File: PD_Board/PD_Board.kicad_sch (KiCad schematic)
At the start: 14 parts

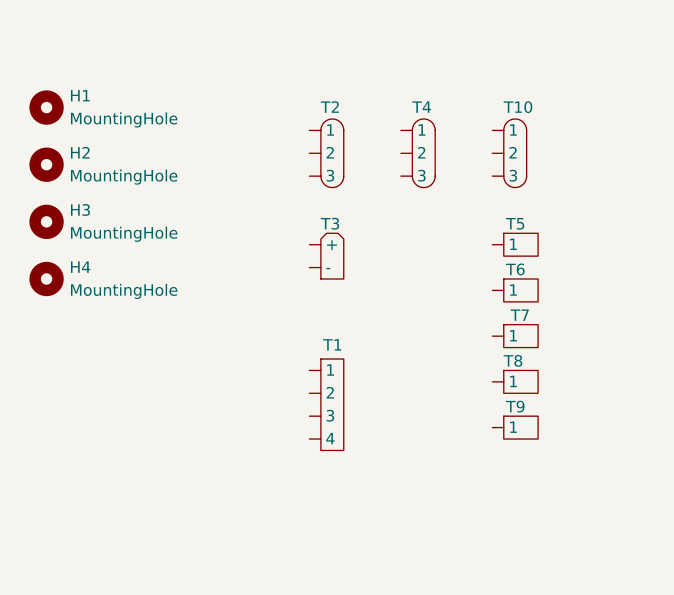
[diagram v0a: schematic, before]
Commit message: started schematic layout
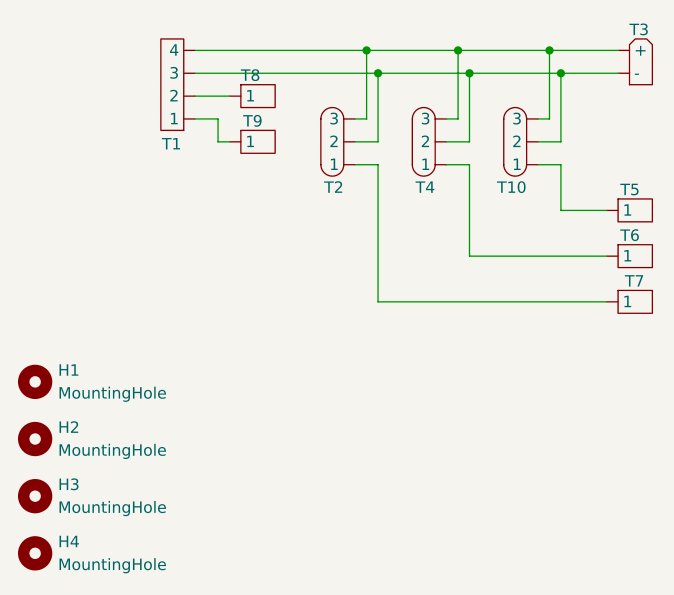
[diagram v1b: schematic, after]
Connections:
- net at T2.1: now also T7.1
- net at T2.2: now also T1.3, T10.2, T3.2 (-), T4.2
- net at T2.3: now also T1.4, T10.3, T3.1 (+), T4.3
- net at T10.1: now also T5.1
- net at T9.1: now also T1.1
- net at T8.1: now also T1.2
- net at T6.1: now also T4.1
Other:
- moved on the sheet: H1, H2, H3, H4, T1, T10, T2, T3, T4, T5, T6, T7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
